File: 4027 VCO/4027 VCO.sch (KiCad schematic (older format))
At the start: 43 parts, among them J18 L.F. CAP, J19 TRIM INPUT, J2 CONT. INPUT, J5 SAW. OUT, J6 POSITIVE SUPPLY, J7 GROUND, J8 NEGATIVE SUPPLY, Q1 2N3906, Q2 2N3904, Q3 2N5459, Q4 2N5459, Q5 2N4125

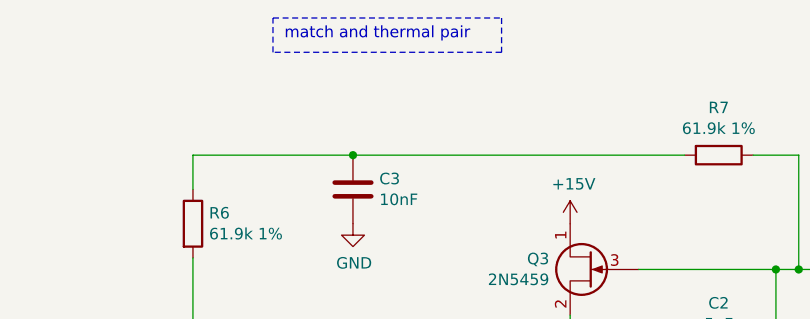
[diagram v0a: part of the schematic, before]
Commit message: various fixes
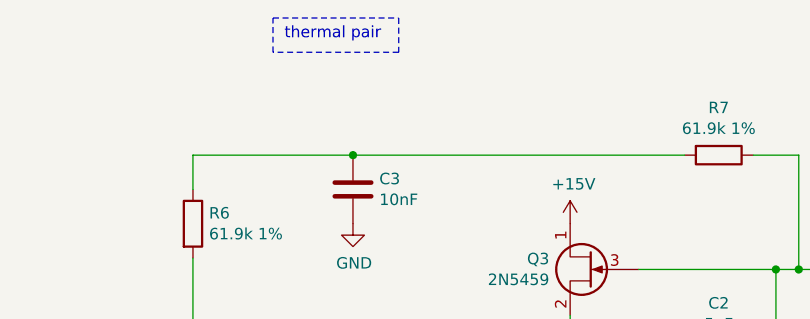
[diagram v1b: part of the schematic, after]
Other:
- note added: "thermal pair"
- note removed: "match and thermal pair"
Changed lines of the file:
@@
 	3650 3850 3650 4150
 Text Notes 3750 1050 0    50   ~ 0
-match and thermal pair
+thermal pair
 Wire Notes Line
-	3700 950  4700 950
+	3700 950  4250 950
 Wire Notes Line
-	4700 950  4700 1100
+	4250 950  4250 1100
 Wire Notes Line
-	4700 1100 3700 1100
+	4250 1100 3700 1100
 Wire Notes Line
 	3700 1100 3700 950
